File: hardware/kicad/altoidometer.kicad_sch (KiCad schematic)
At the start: 27 parts, among them J1 AudioJack3, J1 Conn_01x15_Pin, J2 AudioJack3, SW1 SW_Push, SW2 SW_Push, SW3 SW_Push, SW4 SW_Push, SW5 SW_Push, SW6 SW_Push, SW7 SW_Push, SW8 SW_Push, U1 DOIT-ESP32-DEVKIT-V1, U3 MAX44248ASA+, U4 MICROSD_SPI_OR_SDIO_CARD

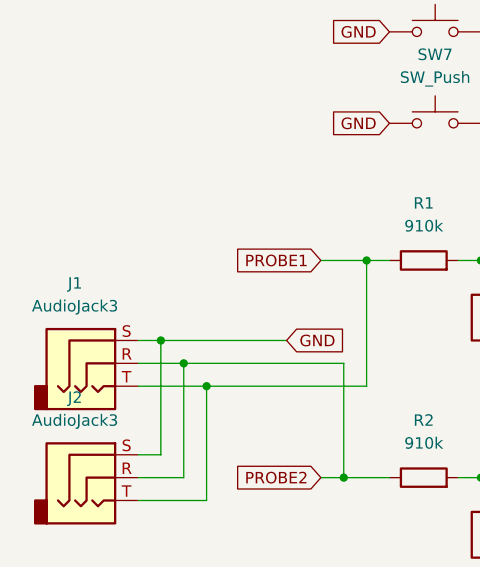
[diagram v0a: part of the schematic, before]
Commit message: idek kicad just did this when i saved
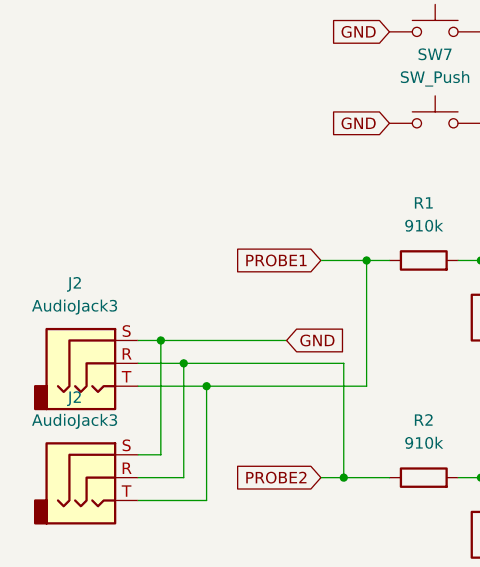
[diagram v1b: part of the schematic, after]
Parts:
- renumbered J1 to J2
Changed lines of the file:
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@@
 	(title_block
 		(title "Altoidometer")
-		(rev "rev1")
+		(rev "1")
 	)
 	(text "expansion pins:\n1. GND\n2. 3V3\n3. I2C SDA\n4. I2C SCL\n5. SPI SCK\n6. SPI MOSI\n7. SPI MISO\n8. SPI CS\n9. UART TX\n10. UART RX\n11. NC\n12. NC\n13. NC\n14. NC\n15. NC"
@@
 		(on_board yes)
 		(dnp no)
-		(fields_autoplaced yes)
 		(property "Reference" "SW1"
 			(at 71.12 24.13 0)
@@
 		(dnp no)
 		(fields_autoplaced yes)
-		(property "Reference" "J1"
+		(property "Reference" "J2"
 			(at 31.115 101.6 0)
 			(effects
@@
 			(project ""
 				(path "/b57712fc-be2e-4ea6-81e8-e743779dbbdf"
-					(reference "J1")
+					(reference "J2")
 					(unit 1)
 				)
